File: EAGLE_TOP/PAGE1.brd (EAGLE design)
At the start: 160 x 160 mm, 101 parts, among them Q1 IRF640, U1 NE555_SOP8, U10 NE556_SOP14, U11 4017_SOP16, U12 4017_SOP16, U13 4518_SMD, U14 4510_DIP, U15 4001_SOP14, U16 4081, U2 4040, U3 4030, U4 4030, U5 LM324, U6 4081_SMD, U7 4017_SOP16, U8 4013_SMD, U9 4013_SMD

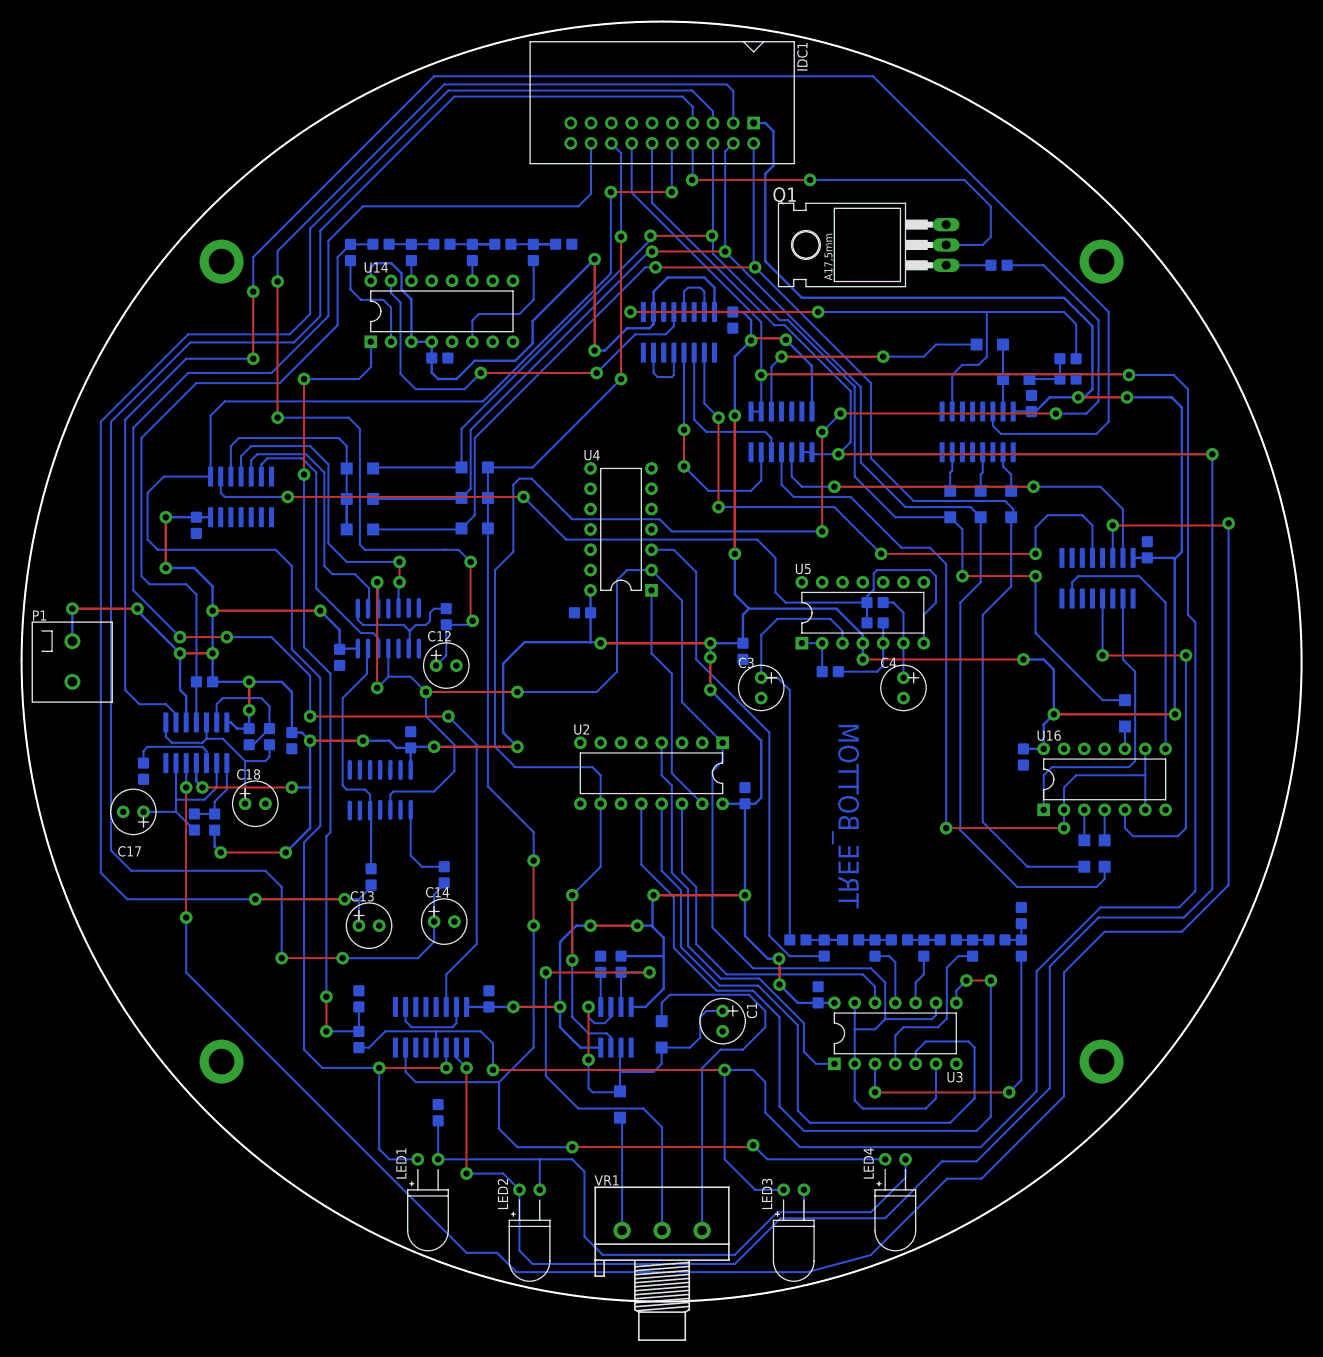
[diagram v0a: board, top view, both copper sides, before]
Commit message: top PCB completed
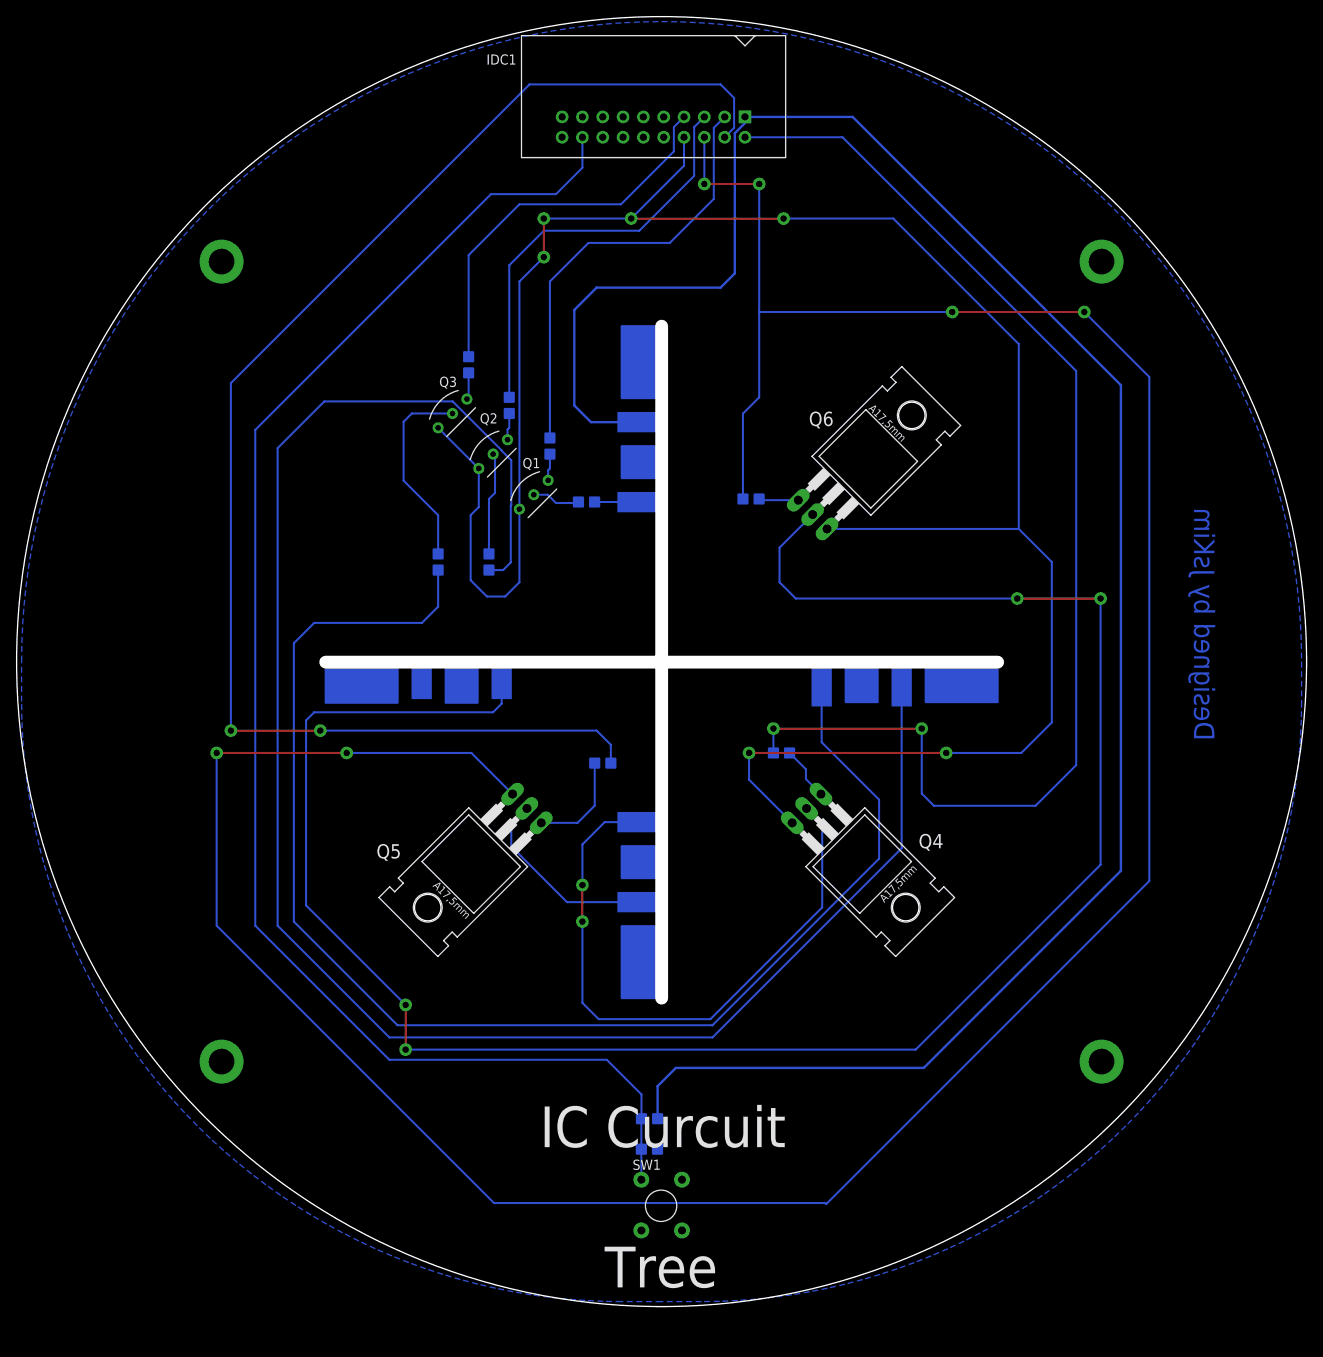
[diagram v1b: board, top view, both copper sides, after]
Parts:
- removed C11, C15, C16, C19, C2, C20, C21, C22, C23, C24, C25, C26, C27, C5, C6, C7, C8, C9: 0.1uF, !JKS:SMD2012
- removed C12, C13, C14, C17, C18, C3: 10uF, !JKS:CAP_POL
- removed C4: 0.012uF, !JKS:CAP_POL
- removed D1, D10, D11, D12, D13, D14, D15, D16, D2, D3, D4, D5, D6, D7, D8, D9: 1N4148, !JKS:SMD_DIODE
- removed LED1, LED2, LED3, LED4: (no value), !JKS:LED_5MM_BEN
- removed P1: (no value), !JKS:POWER_2
- removed R11, R12, R14, R15, R39, R41, R43, R45, R46, R47: 20K, !JKS:SMD2012
- removed R13, R16, R34, R36, R38, R40, R42, R44, R48: 10K, !JKS:SMD2012
- removed R18: 1K, !JKS:SMD2012
- removed R19, R20, R21: 100k, !JKS:SMD2012
- removed R35, R37: 2.2K, !JKS:SMD2012
- removed U1: NE555_SOP8, !JKS:SOP8
- removed U10: NE556_SOP14, !JKS:SOP14
- removed U11, U12, U7: 4017_SOP16, !JKS:SOP16
- removed U13: 4518_SMD, !JKS:SOP16
- removed U14: 4510_DIP, !JKS:DIP16
- removed U15: 4001_SOP14, !JKS:SOP14
- removed U16: 4081, !JKS:DIP14
- removed U2: 4040, !JKS:DIP16
- removed U3, U4: 4030, !JKS:DIP14
- removed U5: LM324, !JKS:DIP14
- removed U6: 4081_SMD, !JKS:SOP14
- removed U8, U9: 4013_SMD, !SEM_03:SOIC_14
- removed VR1: 10K, !JKS:3RP/1610N
- added CON1: TREE_CON, !JKS:TREE_CON
- added Q2, Q3: C1815, !JKS:TO92
- added Q4, Q5, Q6: IRF640, transistor-fet:TO220
- added SW1: (no value), !JKS:PUSH_SW
- C1: value 0.1uF -> 47pF; device !JKS:CAP_POL -> !JKS:SMD2012
- Q1: value IRF640 -> C1815; device transistor-fet:TO220 -> !JKS:TO92
- R10, R8: value 10K -> 1K
- R2: value 1K -> 470k
- R3: value 20K -> 470k
- R4: value 10K -> 470k
- R5: value 20K -> 330
- R6: value 10K -> 220
- R7: value 20K -> 220
- R9: value 20K -> 1K
- moved R4 99.0 mm to (55.9, 118.1), turned to 270 degrees
- moved R3 94.7 mm to (61.0, 113.0), turned to 270 degrees
- moved R7 77.6 mm to (52.1, 91.4)
- moved R6 74.5 mm to (58.4, 91.4), turned to 90 degrees
- moved R5 73.9 mm to (71.6, 99.9), turned to 0 degrees
- moved R2 61.1 mm to (66.0, 108.0), turned to 270 degrees
- moved Q1 57.4 mm to (62.2, 99.1), turned to 315 degrees
- moved R10 57.0 mm to (90.2, 100.3), turned to 180 degrees
- moved R9 40.9 mm to (73.7, 67.3), turned to 0 degrees
- moved R8 28.8 mm to (94.0, 68.6), turned to 180 degrees
- moved R1 20.8 mm to (79.5, 22.9), turned to 0 degrees
- moved C1 20.0 mm to (77.5, 19.1), flipped to the bottom, turned to 180 degrees
- moved IDC1 1.32 mm to (90.4, 148.1)
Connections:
- removed net FASTER_CV: R44.2, R45.2, R47.2, U10.11
- removed net MOD_BREATH: IDC1.10, LED1.1, U6.1, U7.3
- removed net MOD_FAST3: IDC1.12, LED2.1, U15.1, U15.2, U7.2
- removed net MOD_FASTER: C20.1, IDC1.14, LED3.1, U15.8, U15.9, U7.4
- removed net MOD_STATIC: D10.1, D11.1, D9.1, IDC1.16, LED4.1, U7.7
- removed net N$1: D1.1, VR1.1
- removed net N$10: U2.12, U3.8
- removed net N$11: U2.14, U3.12
- removed net N$12: U2.15, U4.1
- removed net N$14: R3.1, U3.3
- removed net N$15: R5.1, U3.4
- removed net N$16: R7.1, U3.10
- removed net N$17: R9.1, U3.11
- removed net N$18: R11.1, U4.3
- removed net N$19: R12.1, R3.2, R4.1
- removed net N$2: R1.2, U1.7, VR1.2
- removed net N$20: R4.2, R5.2, R6.1
- removed net N$21: R6.2, R7.2, R8.1
- removed net N$22: R10.1, R8.2, R9.2
- removed net N$23: R10.2, R11.2, R13.1
- removed net N$24: C3.1, R13.2, U5.3
- removed net N$25: R14.1, U5.1, U5.2
- removed net N$26: R15.2, R16.2, U5.7, U6.2
- removed net N$27: R14.2, R15.1, U5.5
- removed net N$28: C4.1, R16.1, U5.6
- removed net N$29: D3.1, D4.1, D5.1, U6.3
- removed net N$3: D2.2, VR1.3
- removed net N$32: U7.10, U7.15
- removed net N$33: LED1.2, LED2.2, LED3.2, LED4.2, R18.1
- removed net N$34: U6.5, U8.2
- removed net N$35: U6.6, U8.12
- removed net N$36: U6.4, U8.5
- removed net N$37: R19.1, U8.1, U8.9
- removed net N$38: R20.1, U8.13, U9.5
- removed net N$39: U2.1, U3.13, U3.2, U3.6, U3.9, U4.2, U8.11, U8.3, U9.3
- removed net N$4: C2.1, U1.5
- removed net N$40: R21.1, U9.1
- removed net N$5: C1.1, D1.2, D2.1, U1.2, U1.6
- removed net N$58: C17.1, R35.2, U10.2, U10.6
- removed net N$59: R34.2, R35.1, U10.1
- removed net N$6: R2.1, U1.3, U2.10
- removed net N$60: U10.5, U11.14
- removed net N$61: C19.1, U10.3
- removed net N$62: U13.5, U13.7
- removed net N$63: U11.12, U13.2
- removed net N$64: U11.15, U15.3
- removed net N$65: U13.3, U15.5
- removed net N$66: U13.4, U15.6
- removed net N$67: U11.2, U16.1
- removed net N$68: U11.4, U16.5
- removed net N$69: U11.7, U16.8
- removed net N$7: Q1.1, R2.2
- removed net N$70: U15.4, U16.2, U16.6, U16.9
- removed net N$71: D6.1, U16.3
- removed net N$72: D7.1, U16.4
- removed net N$73: D8.1, U16.10
- removed net N$74: R36.2, R37.1, U10.13
- removed net N$75: C18.1, R37.2, U10.12, U10.8
- removed net N$76: C20.2, R48.1, U14.1
- removed net N$77: U10.9, U12.14
- removed net N$78: D12.2, D13.2, U12.15
- removed net N$79: R39.1, U14.6
- removed net N$8: U2.4, U3.1
- removed net N$80: D12.1, U15.10
- removed net N$81: D14.1, U12.2
- removed net N$82: D15.1, U12.4
- removed net N$83: D16.1, U12.7
- removed net N$84: C25.1, D13.1, R38.1
- removed net N$85: U13.13, U13.15
- removed net N$86: R38.2, U12.10, U13.9
- removed net N$87: R41.1, U14.11
- removed net N$88: R43.1, U14.14
- removed net N$89: U13.12, U14.15
- removed net N$9: U2.13, U3.5
- removed net N$90: R45.1, U14.2
- removed net N$91: R39.2, R40.1, R46.1
- removed net N$92: R40.2, R41.2, R42.1
- removed net N$93: R42.2, R43.2, R44.1
- new net LED_ARR1: CON1.5, Q4.2
- new net LED_ARR2: CON1.6, Q5.2
- new net LED_ARR3: CON1.7, Q6.2
- new net N$13: Q4.1, R8.2
- new net N$43: Q5.1, R9.2
- new net N$46: Q6.1, R10.2
- new net N$50: Q1.3, R2.2
- new net N$53: Q2.3, R3.2
- new net N$54: Q3.3, R4.2
- new net N$55: Q1.2, R5.2
- new net N$56: Q2.2, R6.2
- new net N$57: Q3.2, R7.2
- new net RGB_B: CON1.4, R7.1
- new net RGB_G: CON1.3, R6.1
- new net RGB_R: CON1.2, R5.1
- net +5V: now also CON1.1; no longer C11.1, C15.1, C16.1, C21.1, C22.1, C23.1, C24.1, C26.1, C27.1, C5.1, C6.1, C7.1, C8.1, C9.1, P1.1, R34.1, R36.1, R47.1, U1.4, U1.8, U10.10, U10.14, U10.4, U11.16, U12.16, U13.10, U13.16, U14.16, U14.3, U14.4, U15.14, U16.14, U2.16, U3.14, U4.14, U5.4, U6.14, U7.16, U8.14, U9.14
- net GND: now also SW1.P$1; no longer C11.2, C12.2, C13.2, C14.2, C15.2, C16.2, C17.2, C18.2, C19.2, C2.2, C21.2, C22.2, C23.2, C24.2, C25.2, C26.2, C27.2, C3.2, C4.2, C5.2, C6.2, C7.2, C8.2, C9.2, P1.2, Q1.3, R12.2, R18.2, R46.2, R48.2, U1.1, U10.7, U11.13, U11.8, U12.13, U12.8, U13.1, U13.8, U14.10, U14.12, U14.13, U14.5, U14.8, U14.9, U15.7, U16.7, U2.11, U2.8, U3.7, U4.7, U5.11, U6.7, U7.13, U7.8, U8.10, U8.4, U8.6, U8.7, U8.8, U9.4, U9.6, U9.7
- net LED_CON_1: now also R8.1; no longer D14.2, D3.2, D6.2, D9.2
- net LED_CON_2: now also R9.1; no longer D10.2, D15.2, D4.2, D7.2
- net LED_CON_3: now also Q5.3, R10.1; no longer D11.2, D16.2, D5.2, D8.2
- net LED_CON_B: now also R4.1; no longer C14.1, R21.2
- net LED_CON_G: now also R3.1; no longer C13.1, R20.2
- net LED_CON_R: now also R2.1; no longer C12.1, R19.2
- net MAIN_BRIGHT: now also Q1.1, Q2.1, Q3.1, Q4.3, Q6.3; no longer Q1.2
- net MOD_SW: now also C1.1, R1.2, SW1.P$2; no longer U7.14
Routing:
- net +5V: track 728.6 -> 257.5 mm, vias 42 -> 0
- net MOD_FASTER: track 318.5 -> 0.00 mm, vias 4 -> 0
- net MOD_FAST3: track 303.3 -> 0.00 mm, vias 4 -> 0
- net N$60: track 264.4 -> 0.00 mm, vias 4 -> 0
- net LED_ARR3: track 0.00 -> 255.6 mm, vias 0 -> 4
- net N$77: track 233.8 -> 0.00 mm, vias 2 -> 0
- net MAIN_BRIGHT: track 53.1 -> 278.1 mm, vias 2 -> 6
- net RGB_G: track 0.00 -> 224.2 mm
- net MOD_BREATH: track 222.4 -> 0.00 mm, vias 4 -> 0
- net LED_CON_3: track 160.3 -> 376.5 mm, vias 4 -> 6
- net N$39: track 209.2 -> 0.00 mm, vias 4 -> 0
- net MOD_STATIC: track 203.3 -> 0.00 mm, vias 6 -> 0
- net N$6: track 201.9 -> 0.00 mm, vias 6 -> 0
- net RGB_B: track 0.00 -> 171.0 mm
- net LED_CON_B: track 211.8 -> 48.6 mm, vias 2 -> 0
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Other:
- board size 160 x 160 mm -> 161.2 x 161.2 mm
- board text added: "Designed by JsKim"
- board text added: "IC Curcuit"
- board text added: "Tree"
- board text removed: "TREE_BOTTOM"
